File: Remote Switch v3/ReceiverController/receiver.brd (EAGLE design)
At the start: 50 x 42 mm, 38 parts, among them IC1 LNK304, IC2 MCP1703CB, IC3 STM8L101F2, J1 POWER_CONN_4, T1 BT136

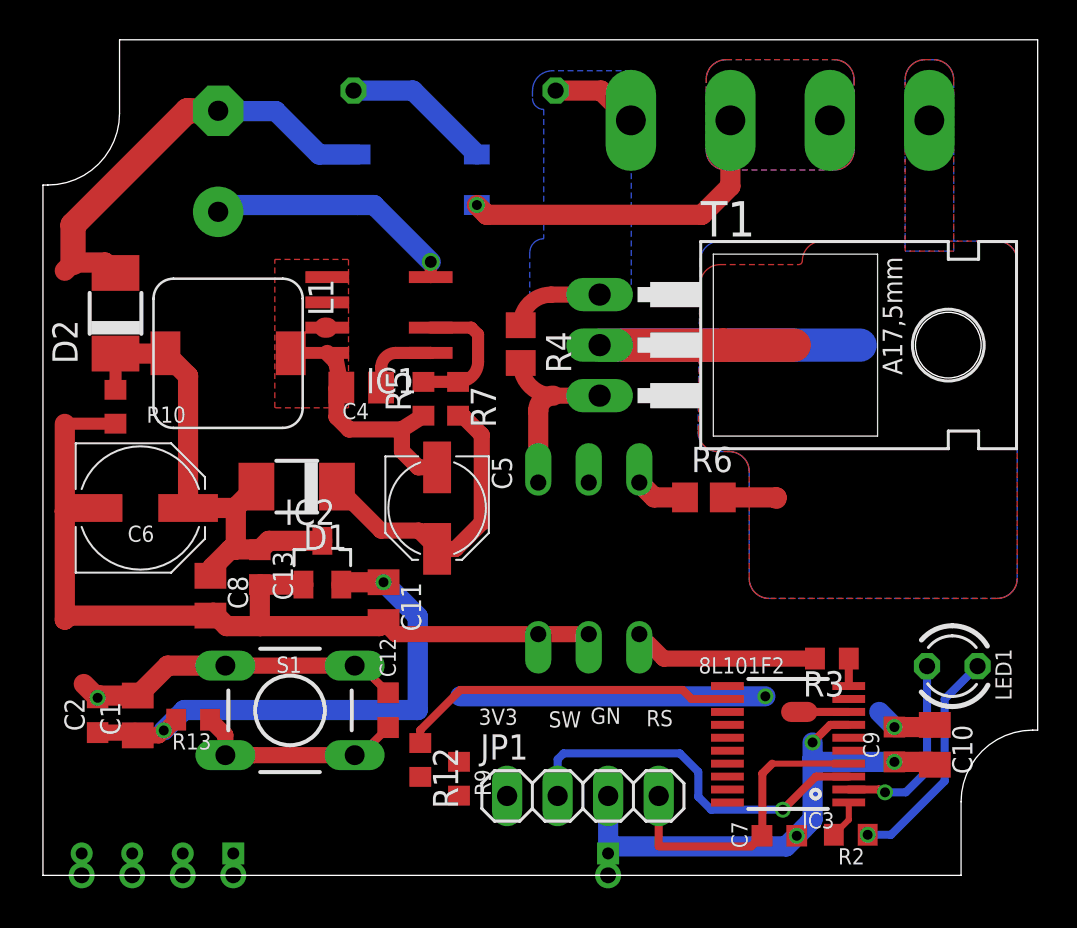
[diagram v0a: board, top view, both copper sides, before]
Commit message: PCB work
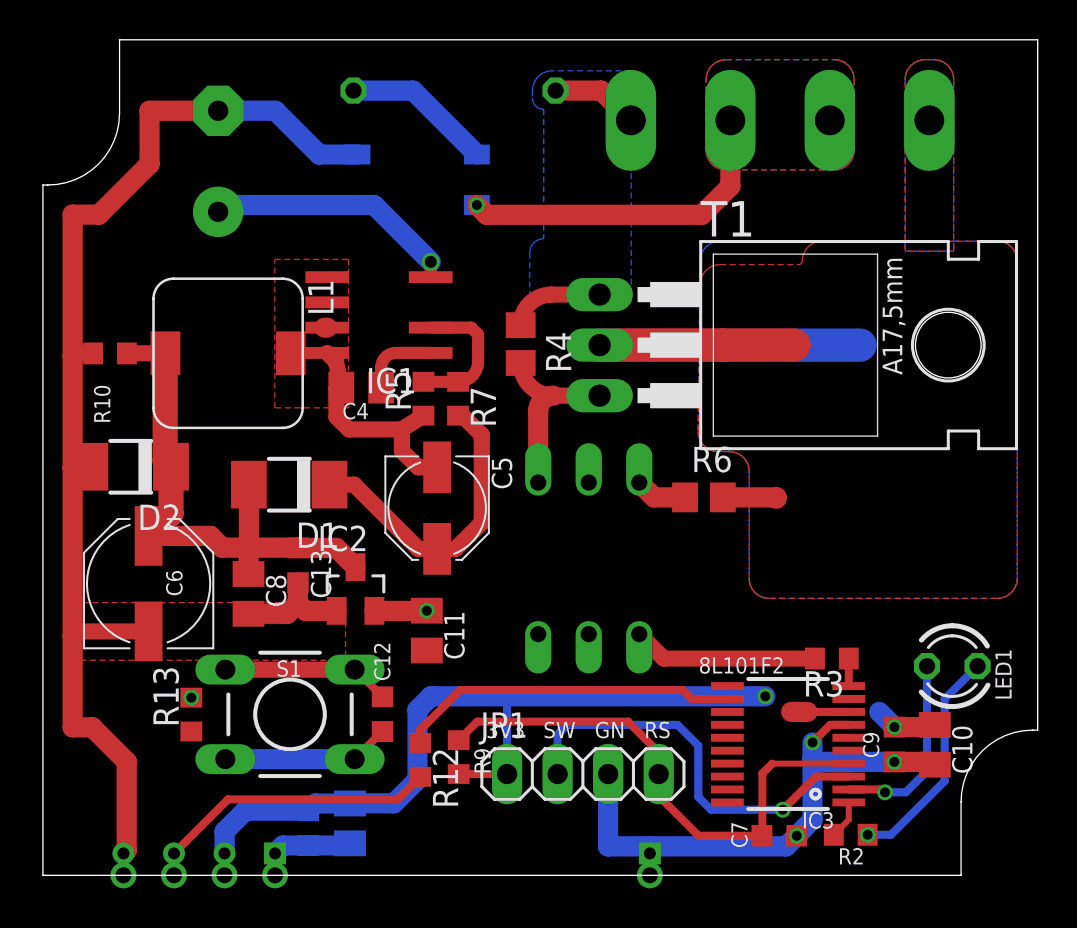
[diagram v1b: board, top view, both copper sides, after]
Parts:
- moved C2 12.0 mm to (13.3, 3.37), flipped to the bottom, turned to 270 degrees
- moved C1 12.0 mm to (15.4, 3.61), flipped to the bottom, turned to 270 degrees
- moved D2 7.75 mm to (4.41, 21.5), turned to 180 degrees
- moved C6 3.83 mm to (5.31, 15.7), turned to 90 degrees
- moved R10 2.69 mm to (3.37, 27.2), turned to 0 degrees
- moved C11 2.61 mm to (19.3, 13.3)
- moved IC2 2.13 mm to (15.7, 15.4)
- moved RF1 2.10 mm to (33.0, 2.10)
- moved C13 1.92 mm to (12.8, 16.6)
- moved C8 1.92 mm to (10.3, 15.1)
- moved JP1 1.10 mm to (27.1, 6.09)
- moved R9 1.09 mm to (20.9, 6.94)
- moved D1 0.39 mm to (12.4, 20.6)
- moved C12 0.34 mm to (17.1, 9.10)
- moved R13 0.27 mm to (7.46, 9.08), turned to 90 degrees
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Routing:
- net RF_DATA: track 0.00 -> 14.0 mm
- net RST: track 15.8 -> 27.1 mm
- net GND: track 110.2 -> 104.2 mm, vias 4 -> 3
- net BTN1: track 10.9 -> 8.48 mm
- net +5V: track 25.3 -> 27.5 mm
- net SWIM: track 19.2 -> 20.8 mm
- added copper zone on layer 1, net GND
